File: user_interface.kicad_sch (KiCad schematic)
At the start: 29 parts, among them J3 Внутр. коннектор потенциометр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, J4 Внутр. коннектор галлетника (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, SW1 Кнопка тактовая 6x6 без фикса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, SW2 Кнопка тактовая 6x6 без фикса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, SW3 Кнопка тактовая 6x6 без фикса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, SW4 Кнопка тактовая 6x6 без фикса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, SW5 Кнопка тактовая 6x6 без фикса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, SW6 Кнопка тактовая 6x6 без фикса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

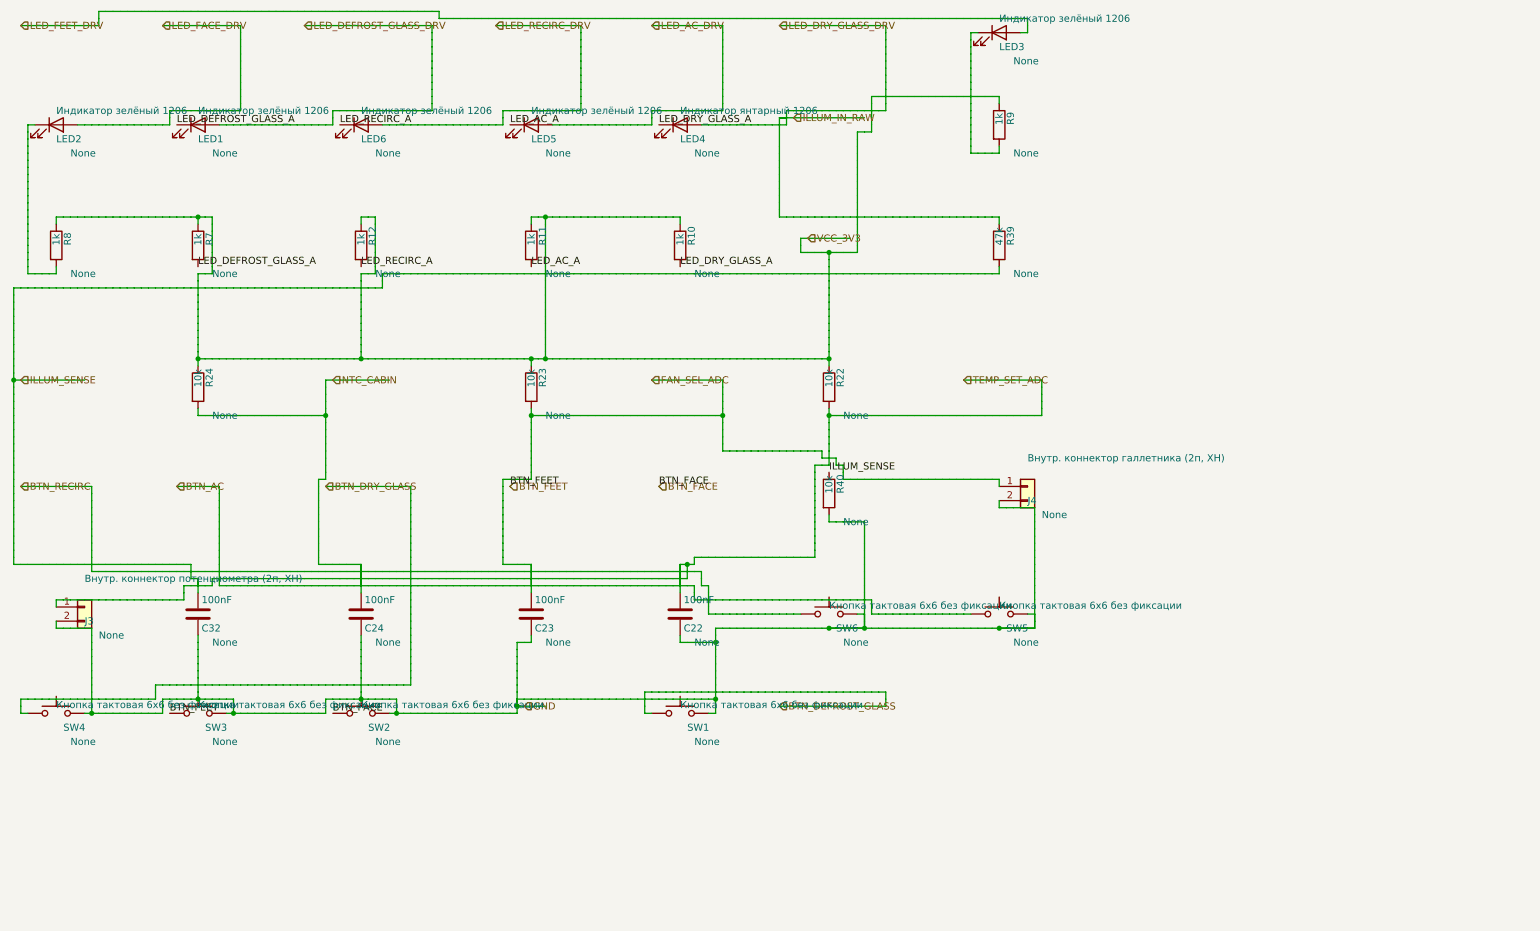
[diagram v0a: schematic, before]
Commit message: рефакторинг проекта и начала прогона тестов
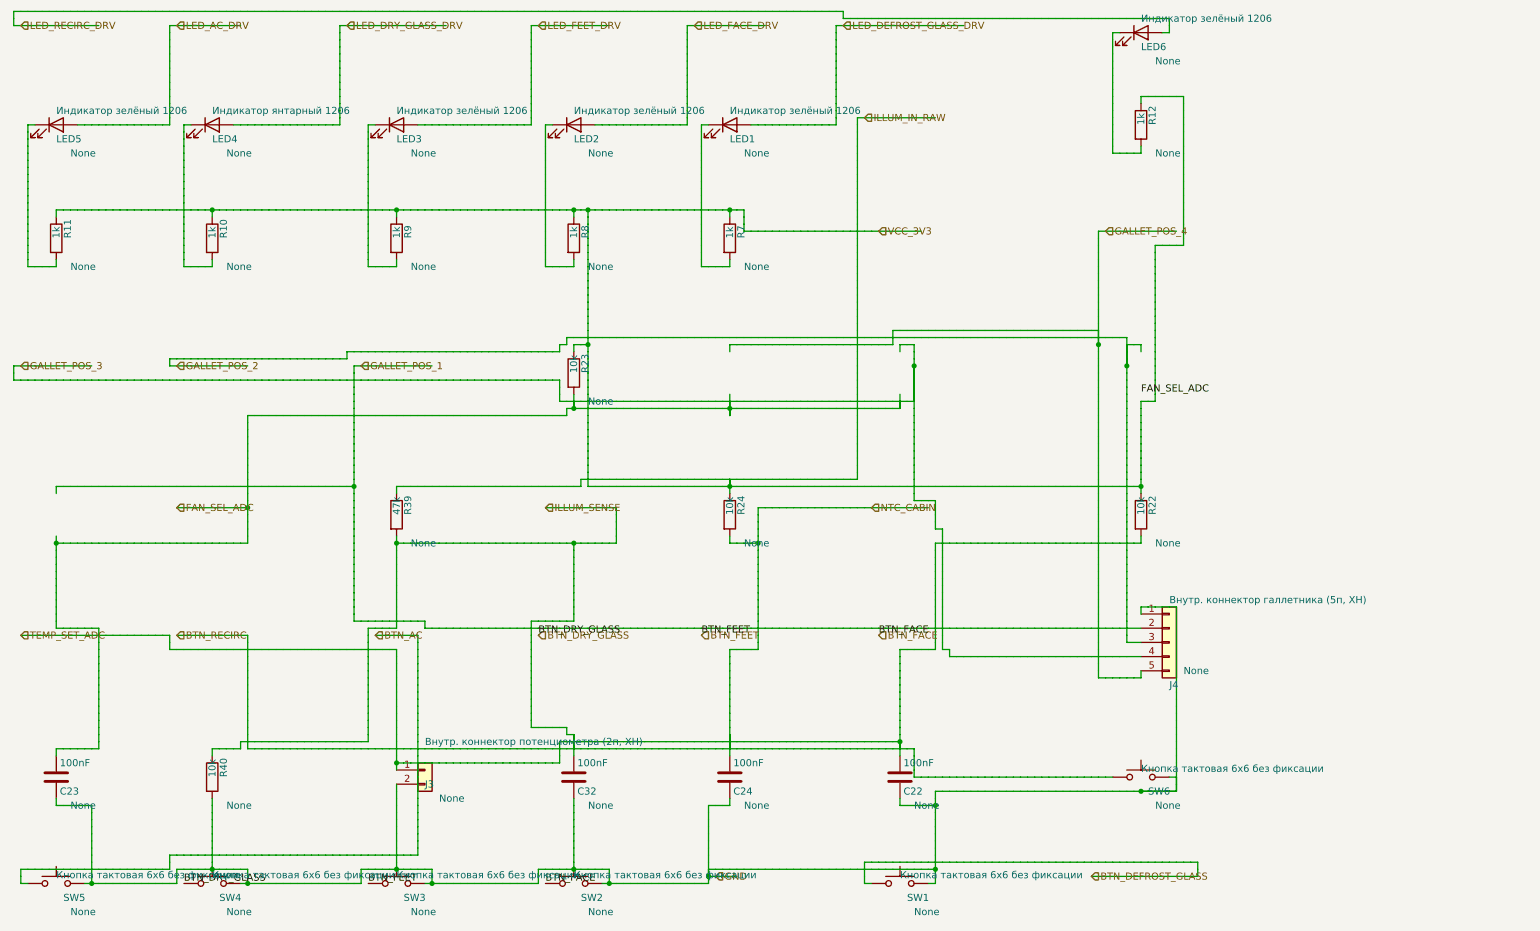
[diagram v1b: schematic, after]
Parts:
- removed J4: Внутр. коннектор галлетника (2п, XH), symbol Connector_Generic:Conn_01x02
- added J4: Внутр. коннектор галлетника (5п, XH), symbol Connector_Generic:Conn_01x05
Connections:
- net LED_DEFROST_GLASS_A is gone; now on net BTN_AC: LED1.1 (K), R7.2
- net LED_DRY_GLASS_A is gone; now on net BTN_AC: LED4.1 (K), R10.2
- net BTN_AC: now also LED2.1 (K), R8.2, J4.1 (Pin_1), J4.2 (Pin_2), J4.3 (Pin_3), J4.4 (Pin_4), J4.5 (Pin_5); no longer LED4.2 (A), SW4.1
- net LED_AC_A: no longer names the net of LED5.1 (K), R11.2
- net LED_RECIRC_A: no longer names the net of LED6.1 (K), R12.2
- new net BTN_DRY_GLASS: SW4.1
- new net LED_DRY_GLASS_DRV: LED4.2 (A)
